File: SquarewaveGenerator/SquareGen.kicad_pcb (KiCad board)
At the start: 2 copper layers, 29.7 x 28.1 mm, 11 parts, among them J1 , J2 , U1 74AC14

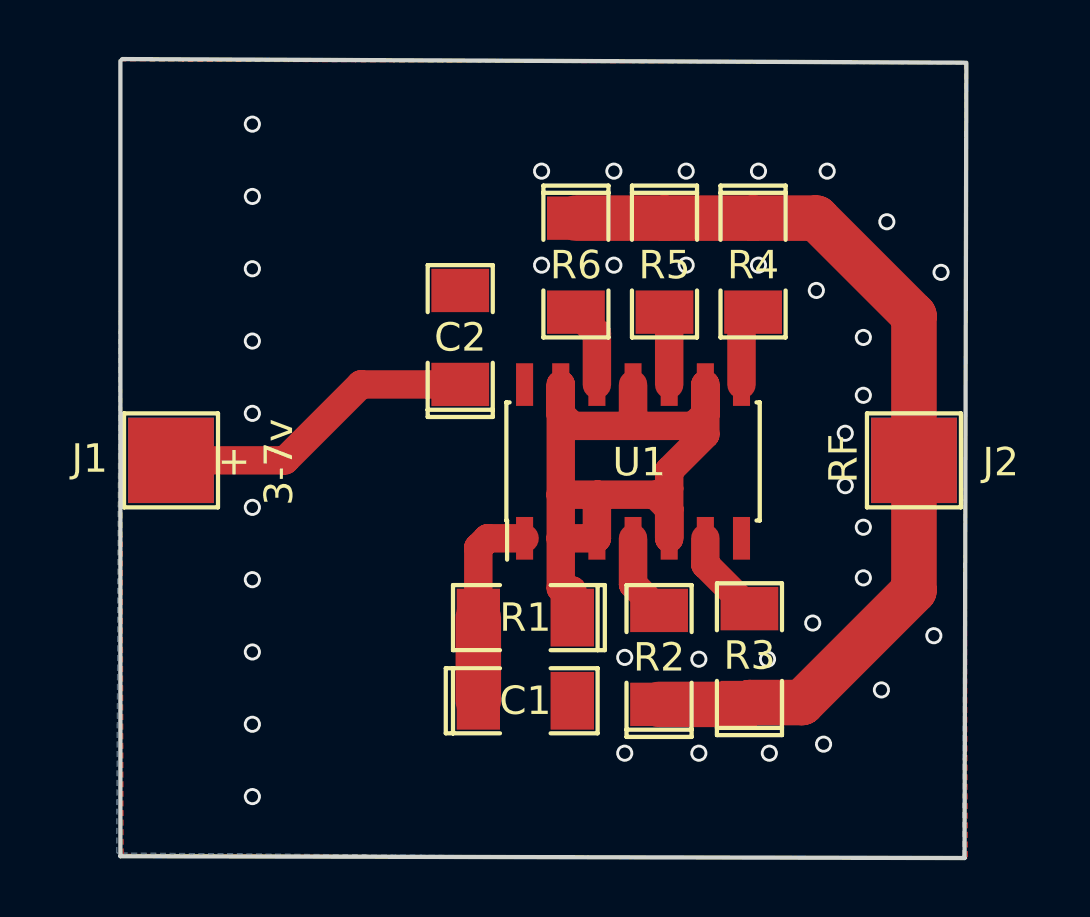
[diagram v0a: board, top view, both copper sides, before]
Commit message: Final update of this project.
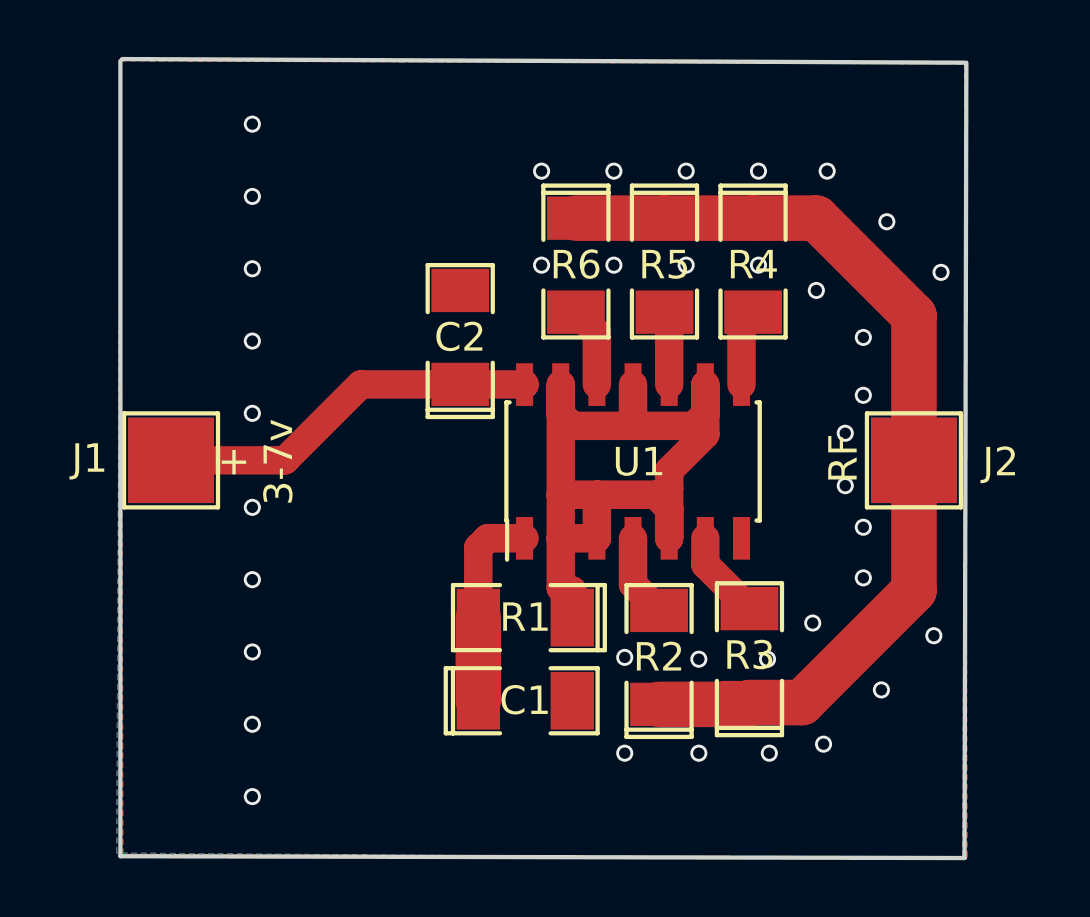
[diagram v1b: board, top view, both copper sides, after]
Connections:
- net /SIG renamed Net-(J2-Pad1)
- U1 pad 14: Net-(U1-Pad14) -> VCC
- U1 pad 7: Net-(U1-Pad7) -> GND
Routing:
- net VCC: track 11.3 -> 13.5 mm
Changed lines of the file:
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@@
     (thickness 1.6)
     (drawings 10)
-    (tracks 93)
+    (tracks 95)
     (zones 0)
     (modules 11)
-    (nets 13)
+    (nets 11)
   )
   (page A4)
@@
   )
   (setup
-    (last_trace_width 1)
+    (last_trace_width 0.25)
     (user_trace_width 1)
     (user_trace_width 1.6)
@@
       (drillshape 0)
       (scaleselection 1)
-      (outputdirectory "/Users/r-w/git/SquareWaveGenerator/gerber/"))
+      (outputdirectory "/Users/r-w/git/KiCad_Projects/SquarewaveGenerator/gerber/"))
   )
   (net 0 "")
@@
   (net 8 "Net-(R5-Pad2)")
   (net 9 "Net-(R6-Pad2)")
-  (net 10 /SIG)
-  (net 11 "Net-(U1-Pad7)")
-  (net 12 "Net-(U1-Pad14)")
+  (net 10 "Net-(J2-Pad1)")
   (net_class Default "This is the default net class."
     (clearance 0.2)
@@
     (uvia_dia 0.3)
     (uvia_drill 0.1)
-    (add_net /SIG)
     (add_net GND)
     (add_net "Net-(C1-Pad1)")
+    (add_net "Net-(J2-Pad1)")
     (add_net "Net-(R1-Pad1)")
     (add_net "Net-(R2-Pad2)")
@@
     (add_net "Net-(R5-Pad2)")
     (add_net "Net-(R6-Pad2)")
-    (add_net "Net-(U1-Pad14)")
-    (add_net "Net-(U1-Pad7)")
     (add_net VCC)
   )
@@
       (net 2 GND))
     (pad 1 smd rect (at 0 0) (size 3 3) (layers F.Cu F.Paste F.Mask)
-      (net 10 /SIG))
+      (net 10 "Net-(J2-Pad1)"))
   )
   (module SquareGen:SOIC-14_3.9x8.7mm_Pitch1.27mm (layer F.Cu)
@@
     (fp_line (start -0.95 -4.35) (end 1.95 -4.35) (layer F.Fab) (width 0.15))
     (pad 14 smd rect (at 2.7 -3.81 90) (size 1.5 0.6) (layers F.Cu F.Paste F.Mask)
-      (net 12 "Net-(U1-Pad14)"))
+      (net 3 VCC))
     (pad 13 smd rect (at 2.7 -2.54 90) (size 1.5 0.6) (layers F.Cu F.Paste F.Mask)
       (net 4 "Net-(R1-Pad1)"))
@@
       (net 7 "Net-(R4-Pad2)"))
     (pad 7 smd rect (at -2.7 3.81 90) (size 1.5 0.6) (layers F.Cu F.Paste F.Mask)
-      (net 11 "Net-(U1-Pad7)"))
+      (net 2 GND))
     (pad 6 smd rect (at -2.7 2.54 90) (size 1.5 0.6) (layers F.Cu F.Paste F.Mask)
       (net 6 "Net-(R3-Pad2)"))
@@
     (fp_line (start -0.889 -1.143) (end -2.54 -1.143) (layer F.SilkS) (width 0.15))
     (pad 1 smd rect (at -1.651 0 90) (size 1.524 2.032) (layers F.Cu F.Paste F.Mask)
-      (net 10 /SIG))
+      (net 10 "Net-(J2-Pad1)"))
     (pad 2 smd rect (at 1.651 0 90) (size 1.524 2.032) (layers F.Cu F.Paste F.Mask)
       (net 5 "Net-(R2-Pad2)"))
@@
     (fp_line (start -0.889 -1.143) (end -2.54 -1.143) (layer F.SilkS) (width 0.15))
     (pad 1 smd rect (at -1.651 0 90) (size 1.524 2.032) (layers F.Cu F.Paste F.Mask)
-      (net 10 /SIG))
+      (net 10 "Net-(J2-Pad1)"))
     (pad 2 smd rect (at 1.651 0 90) (size 1.524 2.032) (layers F.Cu F.Paste F.Mask)
       (net 6 "Net-(R3-Pad2)"))
@@
     (fp_line (start -0.889 -1.143) (end -2.54 -1.143) (layer F.SilkS) (width 0.15))
     (pad 1 smd rect (at -1.651 0 270) (size 1.524 2.032) (layers F.Cu F.Paste F.Mask)
-      (net 10 /SIG))
+      (net 10 "Net-(J2-Pad1)"))
     (pad 2 smd rect (at 1.651 0 270) (size 1.524 2.032) (layers F.Cu F.Paste F.Mask)
       (net 7 "Net-(R4-Pad2)"))
@@
     (fp_line (start -0.889 -1.143) (end -2.54 -1.143) (layer F.SilkS) (width 0.15))
     (pad 1 smd rect (at -1.651 0 270) (size 1.524 2.032) (layers F.Cu F.Paste F.Mask)
-      (net 10 /SIG))
+      (net 10 "Net-(J2-Pad1)"))
     (pad 2 smd rect (at 1.651 0 270) (size 1.524 2.032) (layers F.Cu F.Paste F.Mask)
       (net 8 "Net-(R5-Pad2)"))
@@
     (fp_line (start -0.889 -1.143) (end -2.54 -1.143) (layer F.SilkS) (width 0.15))
     (pad 1 smd rect (at -1.651 0 270) (size 1.524 2.032) (layers F.Cu F.Paste F.Mask)
-      (net 10 /SIG))
+      (net 10 "Net-(J2-Pad1)"))
     (pad 2 smd rect (at 1.651 0 270) (size 1.524 2.032) (layers F.Cu F.Paste F.Mask)
       (net 9 "Net-(R6-Pad2)"))
@@
   (segment (start 140.081 130.2385) (end 143.5735 130.2385) (width 1) (layer F.Cu) (net 3))
   (segment (start 137.414 132.9055) (end 140.081 130.2385) (width 1) (layer F.Cu) (net 3))
+  (segment (start 145.829 130.2385) (end 145.8341 130.2436) (width 1) (layer F.Cu) (net 3))
+  (segment (start 143.5735 130.2385) (end 145.829 130.2385) (width 1) (layer F.Cu) (net 3))
   (segment (start 147.5105 138.43) (end 147.5105 137.4775) (width 1) (layer F.Cu) (net 4))
   (segment (start 147.1041 137.3936) (end 147.1041 135.6436) (width 1) (layer F.Cu) (net 4))
